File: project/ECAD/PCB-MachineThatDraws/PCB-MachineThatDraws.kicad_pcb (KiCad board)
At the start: 2 copper layers, 53.5 x 83 mm, 29 parts, among them J1 SD_Card_Device, J10 Conn_02x03_Odd_Even, J11 Conn_02x03_Odd_Even, J2 SDA/SCL/VCC/GND, J3 Switch, J4 Limit_Switch_X, J5 Moteur, J6 Moteur, J7 Barrel_Jack_Switch, J8 Screw_Terminal_01x02, J9 Servo, U1 ESP32-S3-UNO, U2 R-78E5.0-1.0

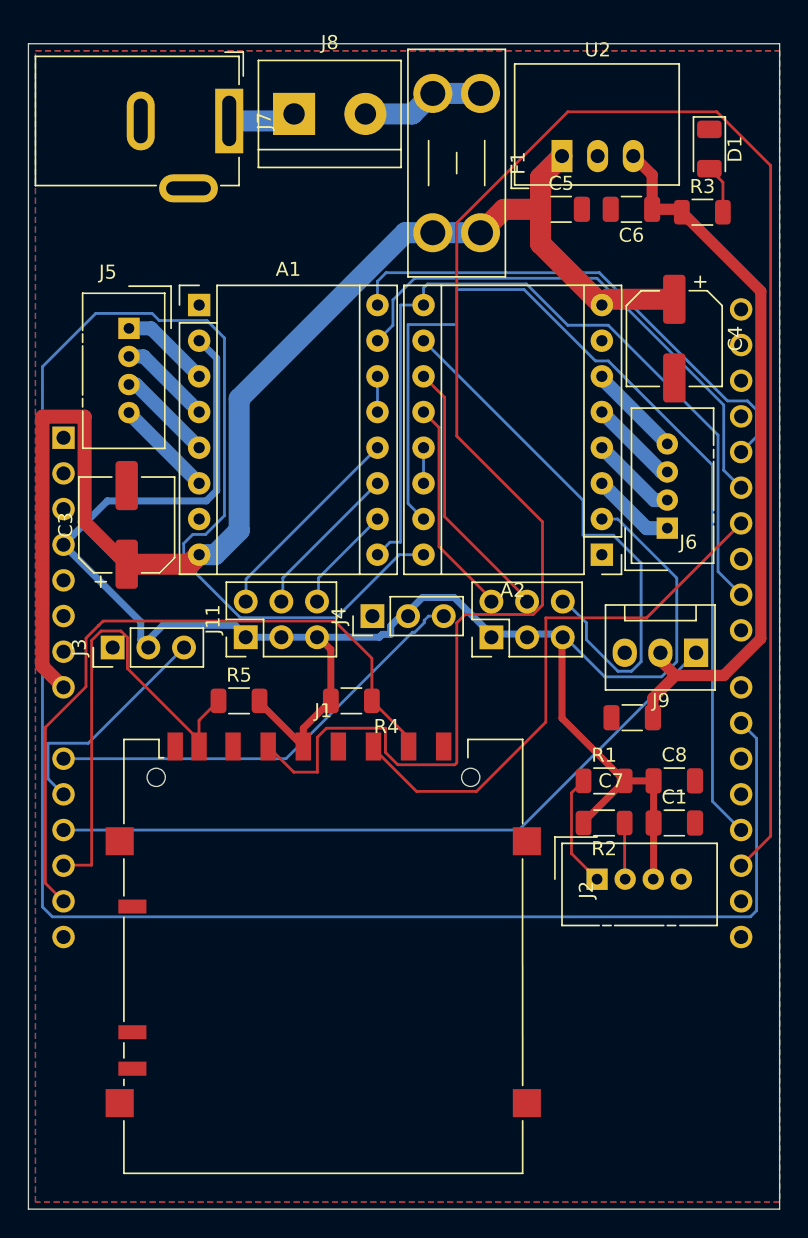
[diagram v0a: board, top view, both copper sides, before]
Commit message: pcb opti
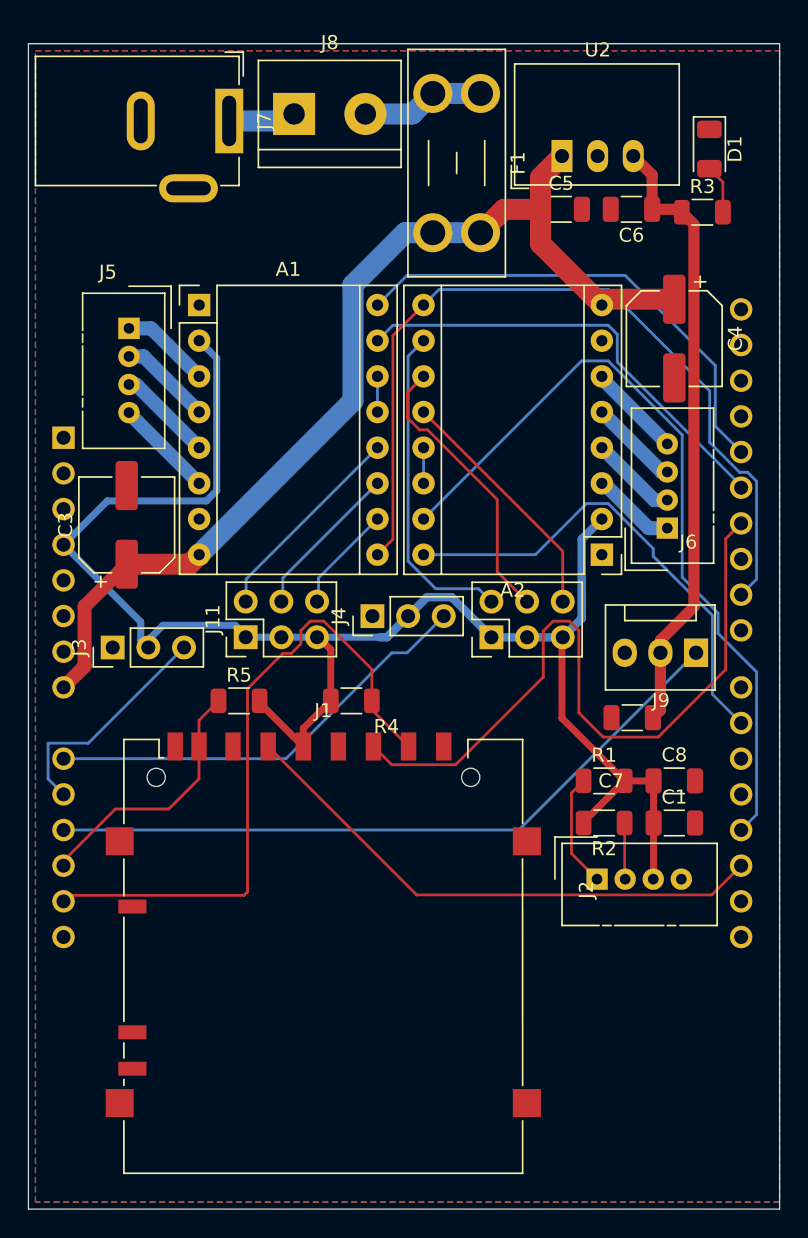
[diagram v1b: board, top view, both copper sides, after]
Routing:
- net D14: track 157.1 -> 34.2 mm
- net D18: track 143.4 -> 38.9 mm
- net +12V: track 98.5 -> 73.8 mm
- net D19: track 34.7 -> 18.5 mm
- net Net-(A2-MS1): track 39.3 -> 23.3 mm
- net D10: track 70.5 -> 56.1 mm
- net +3.3V: track 129.1 -> 115.4 mm
- net D11: track 39.8 -> 51.5 mm
- net +5V: track 52.1 -> 44.1 mm
- net D13: track 37.7 -> 32.4 mm
- net D05: track 49.8 -> 47.3 mm
- net Net-(A2-MS3): track 15.2 -> 17.6 mm
- net D12: track 36.4 -> 34.5 mm
- net Net-(A2-MS2): track 18.8 -> 20.4 mm
